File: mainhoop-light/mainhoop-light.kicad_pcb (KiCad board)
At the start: 2 copper layers, 74 x 69 mm, 79 parts, among them IC1 BCR420U, IC3 BCR420U, IC4 BCR420U, IC5 BCR420U, IC6 BCR420U, J1 Conn_01x04, Q1 2N7002, Q10 Si2301CDS, Q11 2N7002, Q2 Si2301CDS, Q3 2N7002, Q4 2N7002, Q5 Si2301CDS, Q6 2N7002, Q8 2N7002, Q9 2N7002, U1 AP2204K-ADJ, U2 SE555D

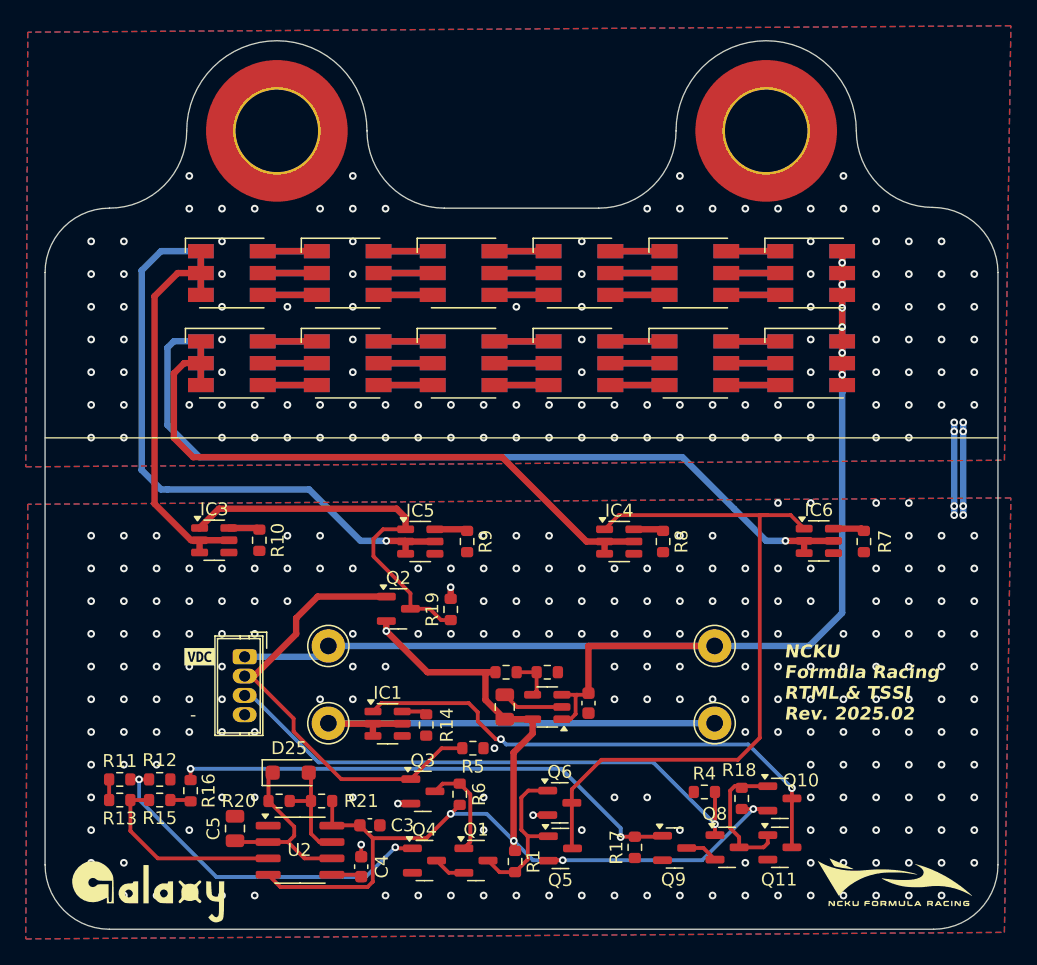
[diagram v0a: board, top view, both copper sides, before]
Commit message: Add files via upload
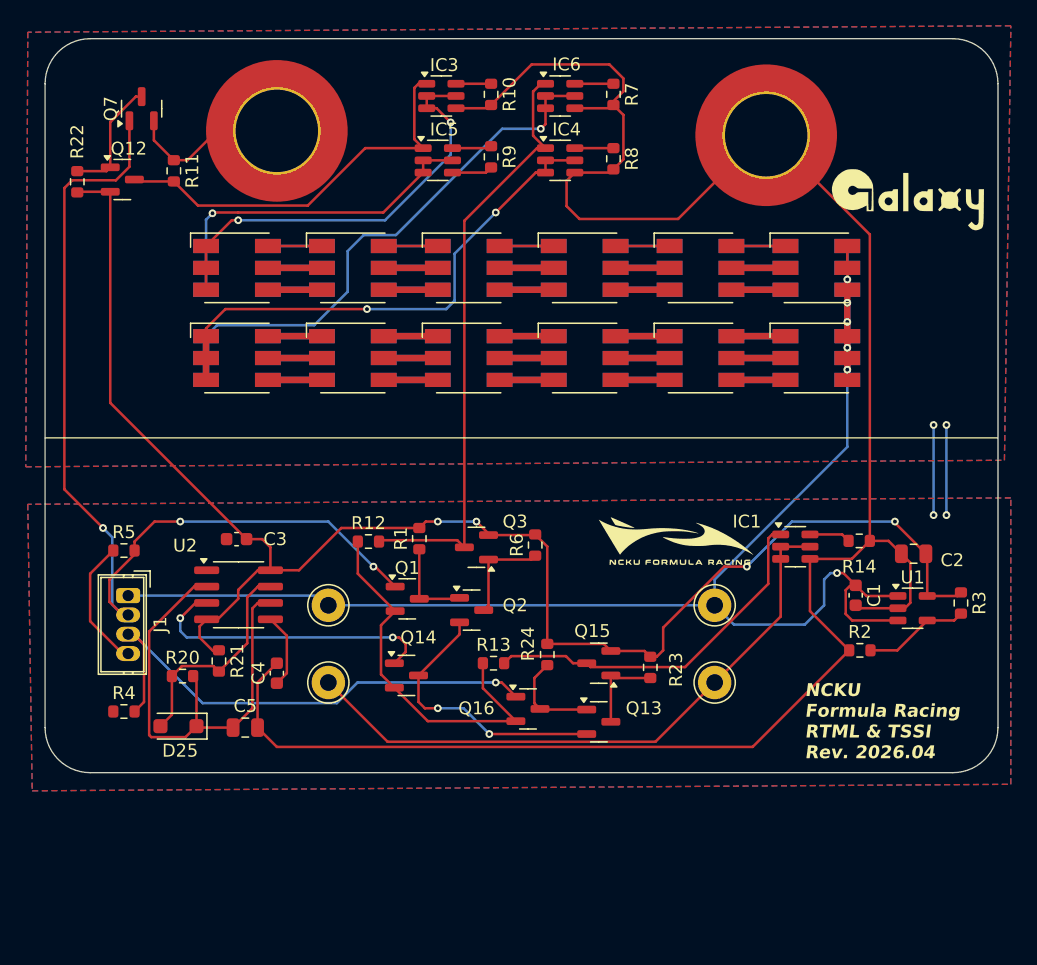
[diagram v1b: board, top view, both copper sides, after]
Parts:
- removed Q10, Q5: Si2301CDS, Package_TO_SOT_SMD:SOT-23
- removed Q11, Q4, Q6, Q8, Q9: 2N7002, Package_TO_SOT_SMD:SOT-23
- removed R15, R16, R17: 1M, Resistor_SMD:R_0603_1608Metric
- removed R18, R19: 100k, Resistor_SMD:R_0603_1608Metric
- removed kibuzzard-67907CEC (x2): G***, kibuzzard-67907CEC
- added Q12: Si2301CDS, Package_TO_SOT_SMD:SOT-23, F.Cu at (68.0, 32.9)
- added Q13: 2N7002, Package_TO_SOT_SMD:SOT-23, F.Cu at (105.0, 75.0)
- added Q14: 2N7002, Package_TO_SOT_SMD:SOT-23, F.Cu at (90.1, 71.5)
- added Q15: Si2301CDS, Package_TO_SOT_SMD:SOT-23, F.Cu at (105.0, 70.5)
- added Q16: 2N7002, Package_TO_SOT_SMD:SOT-23, F.Cu at (99.5, 74.0)
- added Q7: 2N7002, Package_TO_SOT_SMD:SOT-23, F.Cu at (69.5, 27.4)
- added R22: 10k, Resistor_SMD:R_0603_1608Metric, F.Cu at (64.5, 33.1)
- added R23: 10k, Resistor_SMD:R_0603_1608Metric, F.Cu at (109.0, 70.8)
- added R24: 10k, Resistor_SMD:R_0603_1608Metric, F.Cu at (101.0, 69.8)
- Q2: value Si2301CDS -> 2N7002
- Q3: value 2N7002 -> Si2301CDS
- R1, R6: value 100k -> 10k
- R11, R12, R13: value 1M -> 10k
- moved G*** 79.8 mm to (129.0, 34.5)
- moved R11 47.4 mm to (72.0, 32.3), turned to -90 degrees
- moved R4 45.5 mm to (68.1, 74.2)
- moved IC6 40.0 mm to (102.0, 26.4)
- moved R7 39.8 mm to (106.1, 26.3)
- moved R10 39.0 mm to (96.6, 26.3)
- moved IC3 38.7 mm to (92.8, 26.4)
- moved R14 36.5 mm to (125.2, 61.0), turned to 180 degrees
- moved R3 35.7 mm to (133.1, 65.8), turned to -90 degrees
- moved IC1 34.5 mm to (120.3, 61.5)
- moved C2 33.9 mm to (129.4, 62.0), turned to 180 degrees
- moved G*** 31.5 mm to (111.0, 61.0)
- moved R5 31.1 mm to (68.1, 61.8), turned to 0 degrees
- moved R13 30.9 mm to (96.8, 70.5), turned to 0 degrees
- moved R8 30.0 mm to (106.1, 31.3)
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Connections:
- net TSAL renamed RTML
- IC1 pad 1: TSAL_EN -> RTML_EN
- Q1 pad 1: Net-(Q1-G) -> TSSI
- Q1 pad 2: Net-(Q1-S) -> GND
- Q2 pad 1: TSSI -> Net-(Q1-D)
- Q2 pad 2: +12V -> Net-(Q13-S)
- Q2 pad 3: GREEN_EN -> Net-(Q2-D)
- Q3 pad 1: TSSI -> Net-(Q2-D)
- Q3 pad 2: GND -> +12V
- Q3 pad 3: Net-(Q1-G) -> RED_EN
- R1 pad 1: +12V -> Net-(Q1-D)
- R1 pad 2: Net-(Q1-D) -> +12V
- R11 pad 1: Net-(R11-Pad1) -> GND
- R11 pad 2: Net-(Q4-G) -> GREEN_EN
- R12 pad 2: Net-(Q4-G) -> RED_EN
- R13 pad 1: Net-(U2-Q) -> GND
- R13 pad 2: Net-(R11-Pad1) -> RTML_EN
- R4 pad 1: GND -> +5V
- R6 pad 1: +12V -> Net-(Q2-D)
- R6 pad 2: Net-(Q1-G) -> +12V
- U2 pad 3: Net-(U2-Q) -> Net-(Q14-G)
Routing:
- net GND: track 23.2 -> 235.8 mm, vias 336 -> 4
- net TSAL_EN: track 40.6 -> 0.00 mm, vias 2 -> 0
- net Net-(Q9-G): track 40.2 -> 0.00 mm, vias 2 -> 0
- net TSSI: track 36.1 -> 75.5 mm, vias 0 -> 3
- net +12V: track 93.6 -> 122.2 mm, vias 5 -> 4
- net RTML_EN: track 0.00 -> 28.4 mm
- net Net-(Q4-G): track 27.7 -> 0.00 mm, vias 2 -> 0
- net Net-(D14-BK): track 68.6 -> 42.9 mm
- net Net-(Q14-G): track 0.00 -> 23.3 mm, vias 0 -> 2
- net Net-(D7-BK): track 50.1 -> 27.0 mm
- net THR: track 14.6 -> 36.4 mm
- net Net-(Q13-S): track 0.00 -> 21.6 mm, vias 0 -> 2
- net Net-(U2-Q): track 15.4 -> 0.00 mm
- net Net-(IC1-OUT_1): track 36.7 -> 48.8 mm
- net Net-(Q10-G): track 10.7 -> 0.00 mm
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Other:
- board size 74 x 69 mm -> 74 x 57 mm
- board text added: "NCKU Formula Racing RTML & TSSI Rev. 2026.04"
- board text removed: "-"
- board text removed: "NCKU Formula Racing RTML & TSSI Rev. 2025.02"
- board text removed: "R=6.0"
- board text removed: "R=7.0"
